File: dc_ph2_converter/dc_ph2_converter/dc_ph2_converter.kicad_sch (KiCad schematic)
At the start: 3 parts, among them J1 Barrel_Jack_MountingPin, J2 Conn_01x02

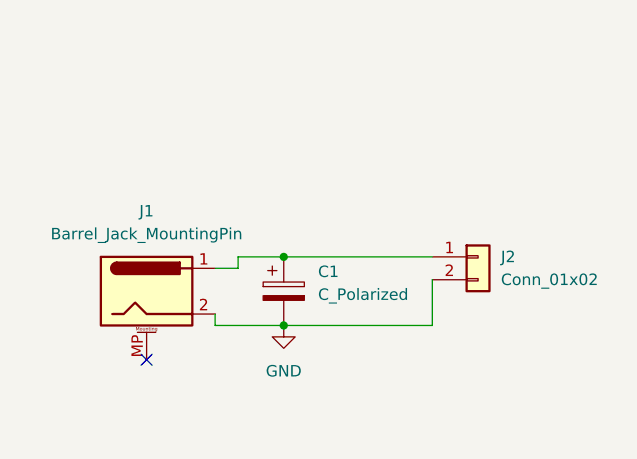
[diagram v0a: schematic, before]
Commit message: Add projects
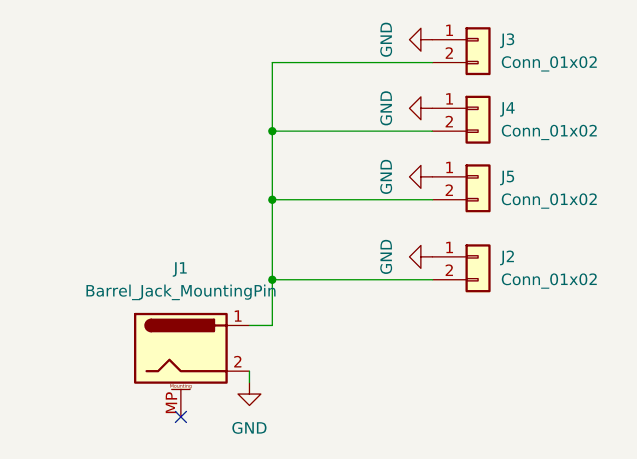
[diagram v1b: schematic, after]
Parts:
- removed C1: C_Polarized, Capacitor_THT:CP_Radial_D12.5mm_P5.00mm, symbol Device:C_Polarized
- added J3, J4, J5: Conn_01x02, Connector_JST:JST_PH_B2B-PH-K_1x02_P2.00mm_Vertical, symbol Connector_Generic:Conn_01x02
- J2: footprint Connector_PinHeader_2.00mm:PinHeader_1x02_P2.00mm_Vertical -> Connector_JST:JST_PH_B2B-PH-K_1x02_P2.00mm_Vertical
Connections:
- net GND: now also J2.1 (Pin_1), J3.1 (Pin_1), J4.1 (Pin_1), J5.1 (Pin_1); no longer J2.2 (Pin_2)
- net at J1.1: now also J2.2 (Pin_2), J3.2 (Pin_2), J4.2 (Pin_2), J5.2 (Pin_2); no longer J2.1 (Pin_1)
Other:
- moved on the sheet: J1
